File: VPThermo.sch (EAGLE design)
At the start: 54 parts, among them SW1 SPST_TACT-KMR2, SW2 SPST_TACT-KMR2, U1 REG1117, U2 ESP-12F, U3 MCP41010-I/SN, U4 RT6208GE, U5 SN74LVC1G3157DBVR, X1 5 x Screw clamp

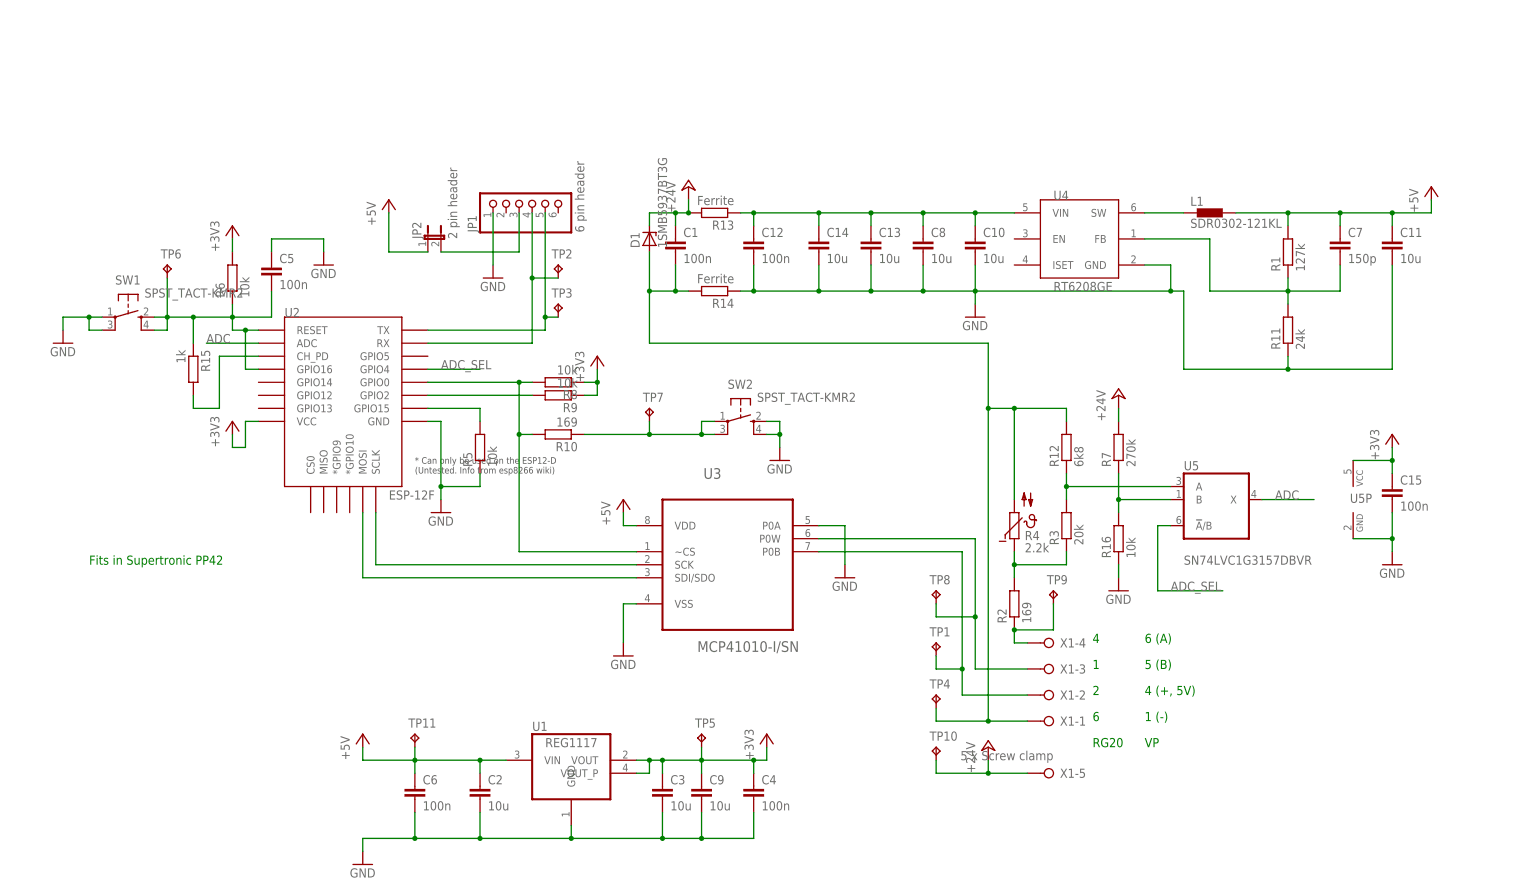
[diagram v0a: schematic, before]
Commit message: Revision C
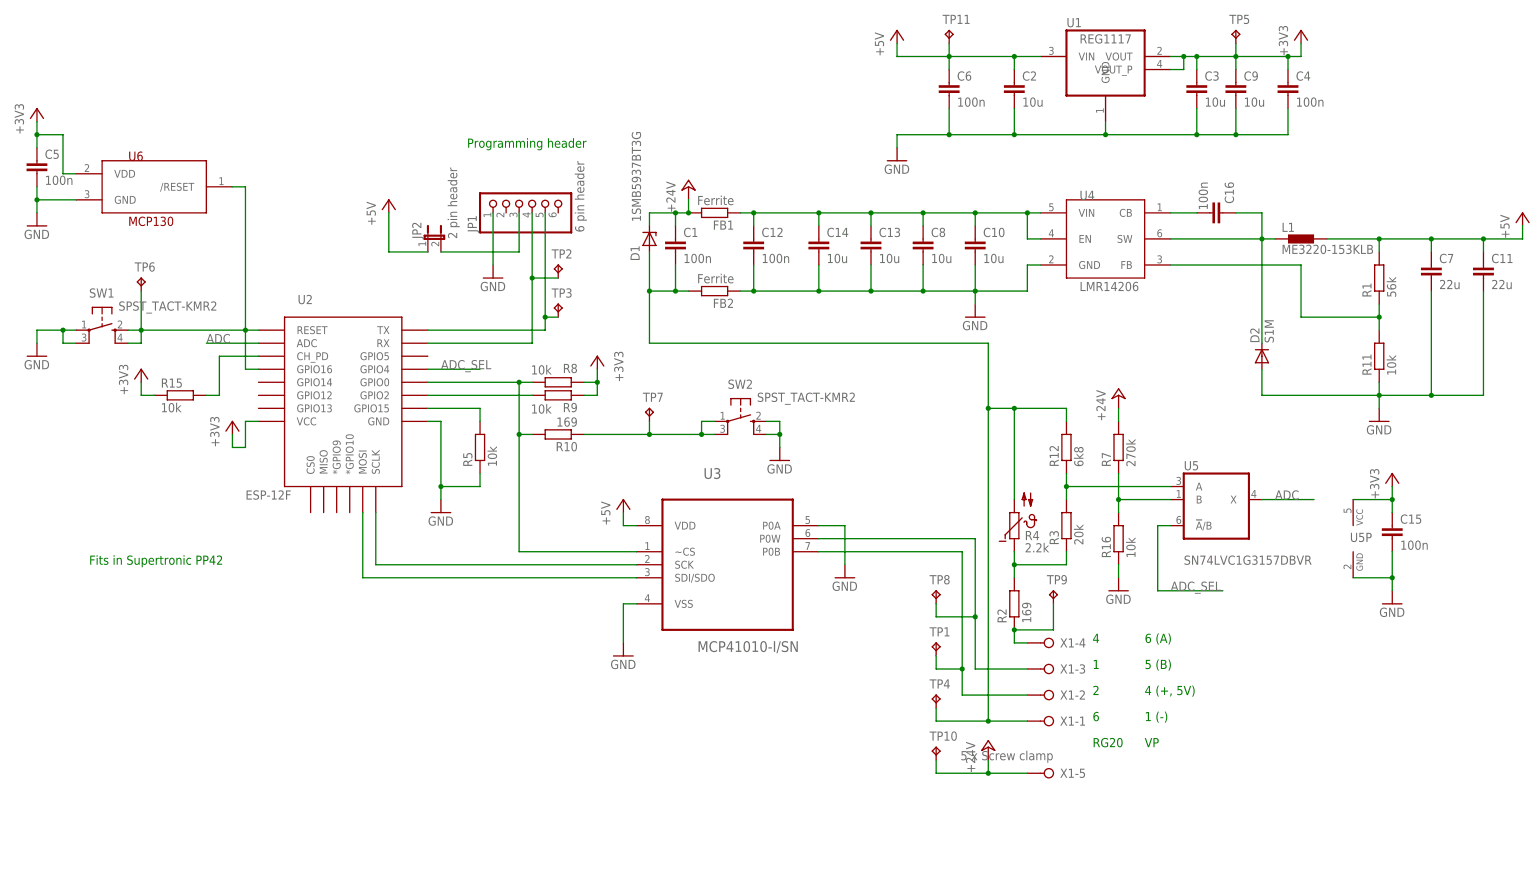
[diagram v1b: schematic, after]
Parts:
- removed R6: 10k, eagle-ltspice:RR0603
- added C16: 100n, rcl:C-EUC0603
- added D2: S1M, diode:S1M
- added U6: MCP130, ola-microchip:MCP130
- C11: value 10u -> 22u; OC_FARNELL 2611943 -> 2309030
- C7: value 150p -> 22u; device rcl:C-EUC0603 -> resistor:C-EUC0805; OC_FARNELL 1759122 -> 2309030
- L1: value SDR0302-121KL -> ME3220-153KLB; OC_FARNELL 2328671 -> 2287926
- R1: value 127k -> 56k; OC_FARNELL 2689436 -> 2303215
- R11: value 24k -> 10k; OC_FARNELL 2447308 -> 2447230
- R15: value 1k -> 10k; OC_FARNELL 2447272 -> 2447230
- R16, R5, R8, R9: OC_FARNELL 2074167 -> 2447230
- U4: value RT6208GE -> LMR14206; device richtek:RT6208GE -> ola_texas:LMR14206; OC_FARNELL 2545963 -> (none)
- renumbered R13 to FB1, R14 to FB2
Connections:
- removed net N$8: C5.2, R15.1, R6.1, SW1.S, SW1.S1, TP6.TP, U2.GPIO16, U2.RESET
- new net N$22: SW1.S, SW1.S1, TP6.TP, U2.GPIO16, U2.RESET, U6./RESET
- new net N$23: C16.1, D2.C, L1.1, U4.SW
- net +3V3: now also C5.1, R15.1, U6.VDD; no longer R6.2
- net GND: now also C5.2, C7.2, D2.A, U6.GND; no longer C5.1
- net N$14: now also U4.EN
- net N$19: no longer C7.2
- net N$3: now also C16.2, U4.CB; no longer L1.1, U4.SW
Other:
- note added: "Programming header"
- moved on the sheet: C11, C15, C2, C3, C4, C5, C6, C7, C9, L1, R1, R11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
